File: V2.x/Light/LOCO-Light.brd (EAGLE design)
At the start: 43.2 x 34.3 mm, 54 parts, among them IC1 Atmega 328-P, IC2 MCP2515, IC3 ACS712ELCTR-20A-T, IC5 LM340MP-05, J1 3-794618-4, J2 3-794618-4, Q1 8MHz, Q2 16MHz, Q3 FDS5680, Q4 FDS5680, Q5 FDS5680, Q6 FDS5680, Q7 FDS5680, Q8 FDS5680, X1 22-23-2081

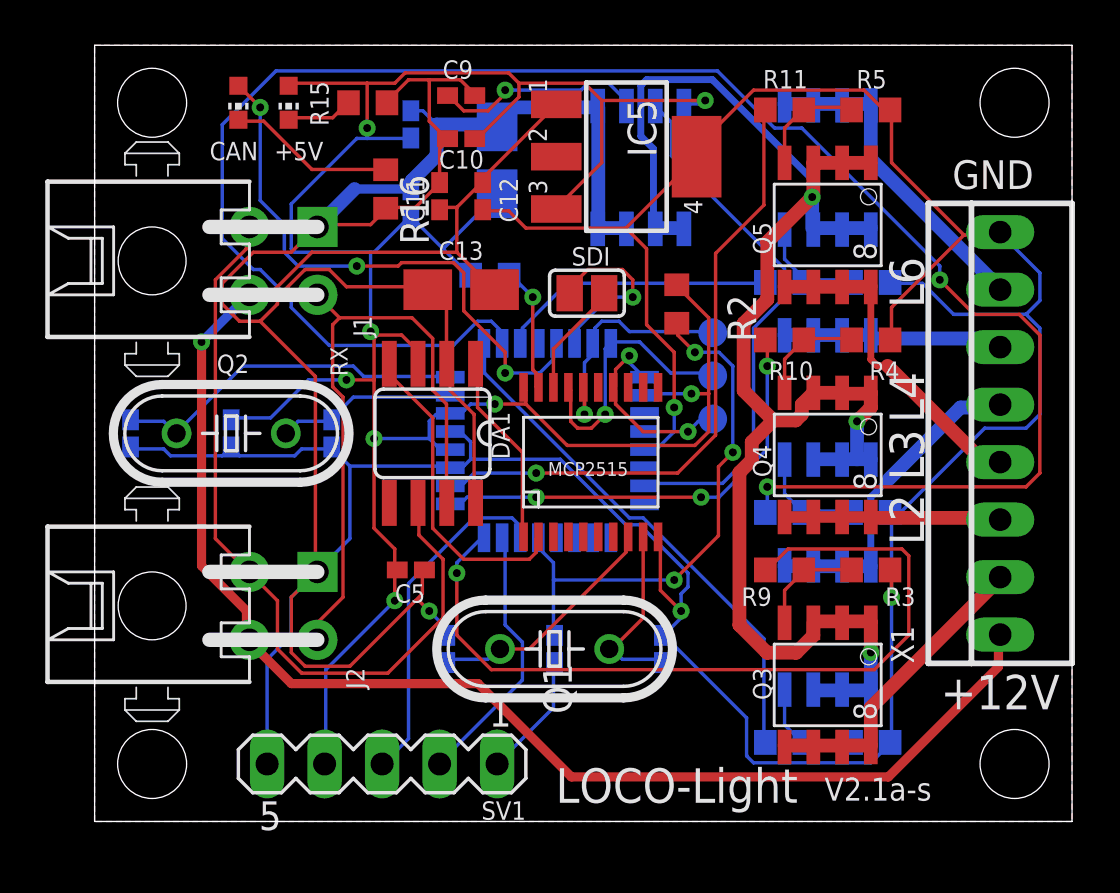
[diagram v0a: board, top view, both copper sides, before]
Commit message: initial
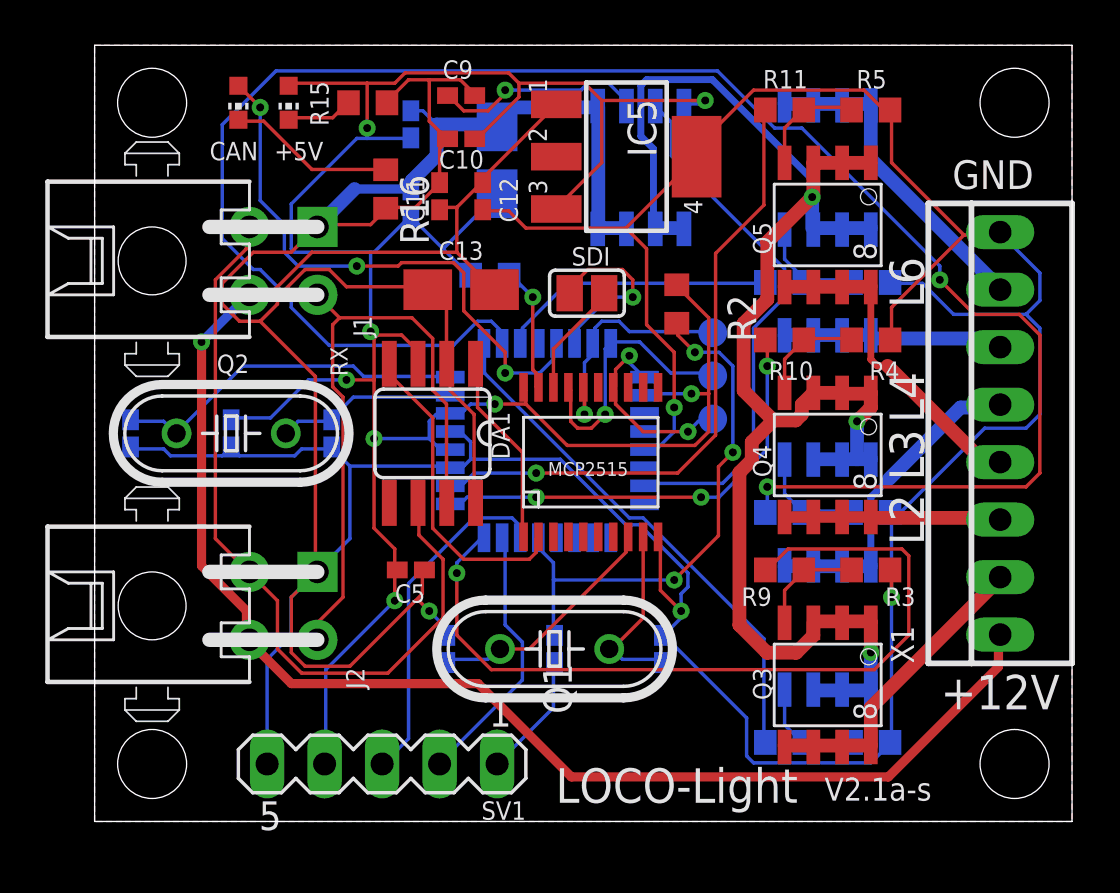
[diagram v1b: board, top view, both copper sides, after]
